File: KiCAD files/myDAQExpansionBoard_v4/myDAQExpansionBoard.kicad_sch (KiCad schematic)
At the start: 73 parts, among them J1 Conn_01x05_Male, J2 Conn_01x05_Male, J3 Conn_01x08_Male, J4 OSTV7XX3151, J5 Screw_Terminal_01x02, J6 Screw_Terminal_01x02, J7 Screw_Terminal_01x01, J8 Screw_Terminal_01x01, SW1 SW_SPDT, SW2 SW_SPDT, SW3 SW_Push, SW4 SW_Push, U1 74LS47, U2 7segm-symbol, U3 ACS712xLCTR-05B, U4 L298N

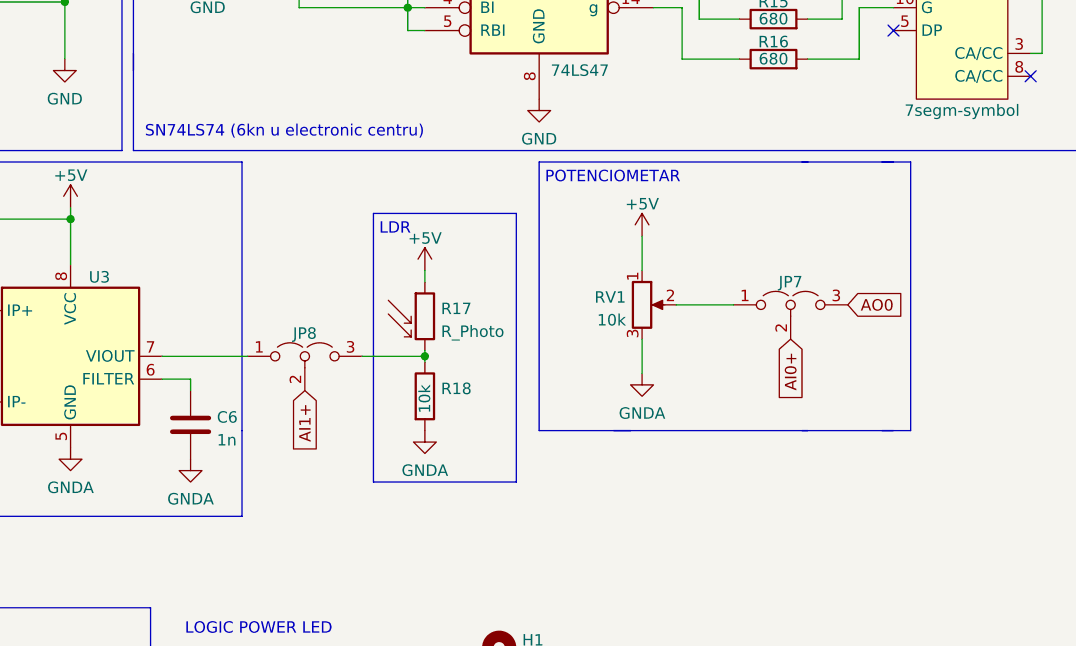
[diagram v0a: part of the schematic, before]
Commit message: update
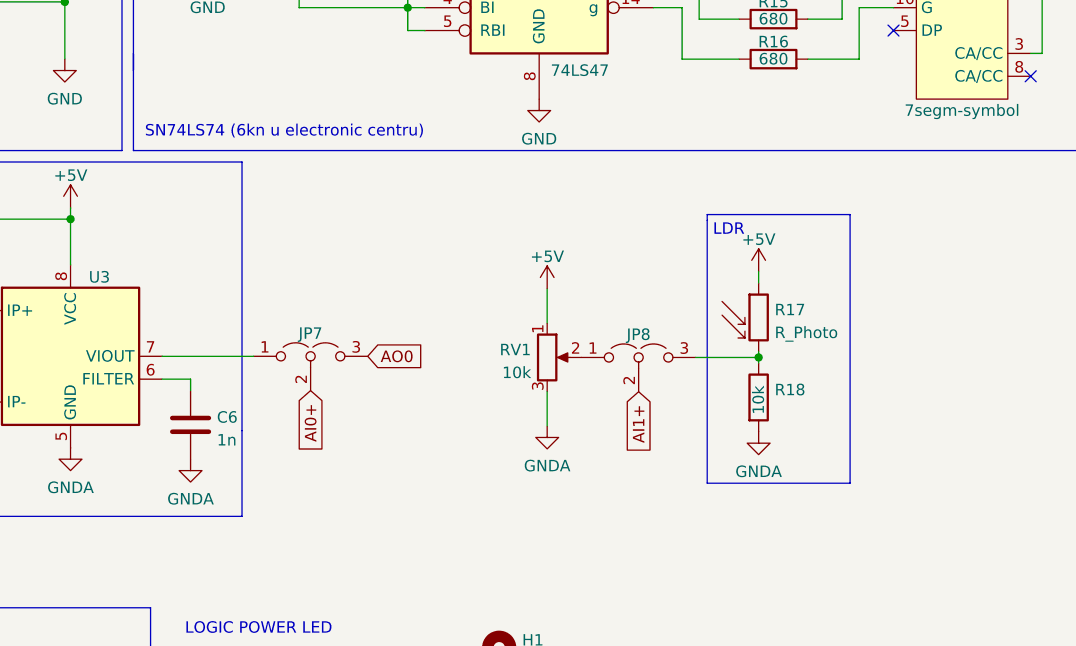
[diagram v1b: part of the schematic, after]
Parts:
- C5: footprint Capacitor_THT:CP_Radial_D12.5mm_P5.00mm -> Capacitor_THT:C_Radial_D10.0mm_H16.0mm_P5.00mm
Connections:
- net at JP8.1 (A): now also RV1.2; no longer U3.7 (VIOUT)
- net at JP7.1 (A): now also U3.7 (VIOUT); no longer RV1.2
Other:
- note removed: "POTENCIOMETAR"
- moved on the sheet: JP7, JP8, R17, R18, RV1
